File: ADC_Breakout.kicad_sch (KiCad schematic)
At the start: 38 parts, among them J0 Conn_01x06, J10 Conn_01x02, J11 Conn_01x02, J12 Conn_01x02, J13 Conn_01x02, J2 Digital Power, J3 Clock Chooser, J4 Analog Power, J6 Conn_01x02, J7 Conn_01x02, J8 Conn_01x02, J9 Conn_01x02, SW1 SW_MEC_5E, U2 SN74AUP2G80DCUR, X1 SIT8924BA-22-33E-8.192000, Y1 Crystal_Small

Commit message: Updated footprint.
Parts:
- D0: footprint Capacitor_SMD:C_0603_1608Metric_Pad1.08x0.95mm_HandSolder -> TVS:VAR_CG0603MLU-3.3E
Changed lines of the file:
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@@
 			)
 		)
-		(property "Footprint" "Capacitor_SMD:C_0603_1608Metric_Pad1.08x0.95mm_HandSolder"
+		(property "Footprint" "TVS:VAR_CG0603MLU-3.3E"
 			(at 38.1 88.9 0)
 			(effects

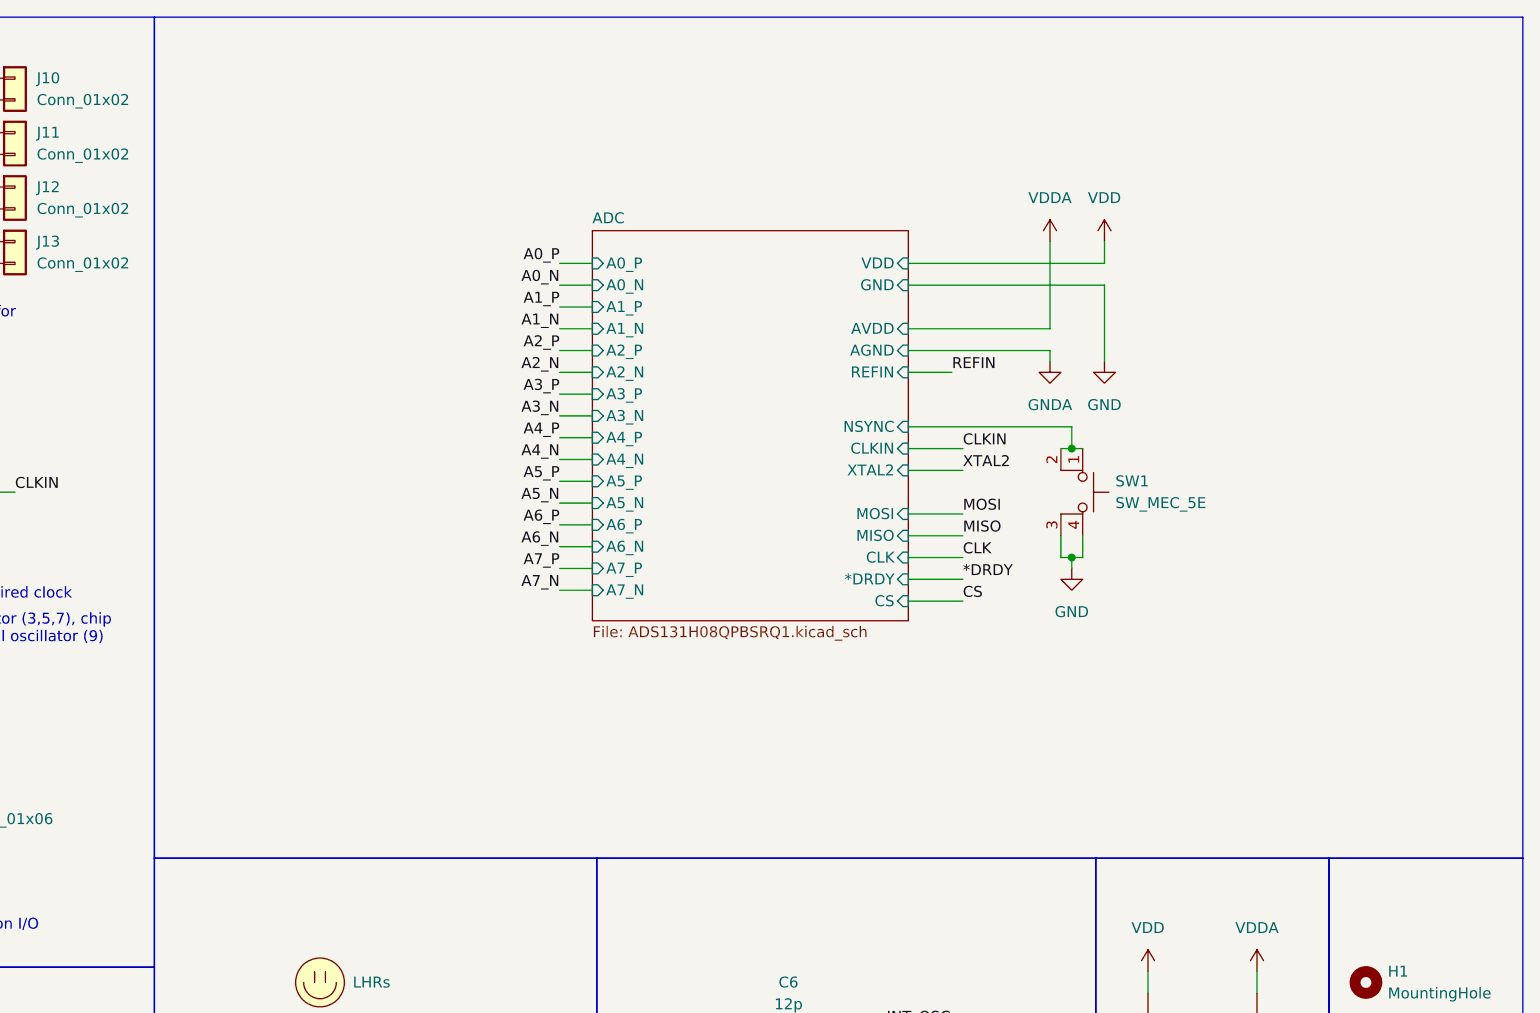
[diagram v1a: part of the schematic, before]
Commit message: gerebres
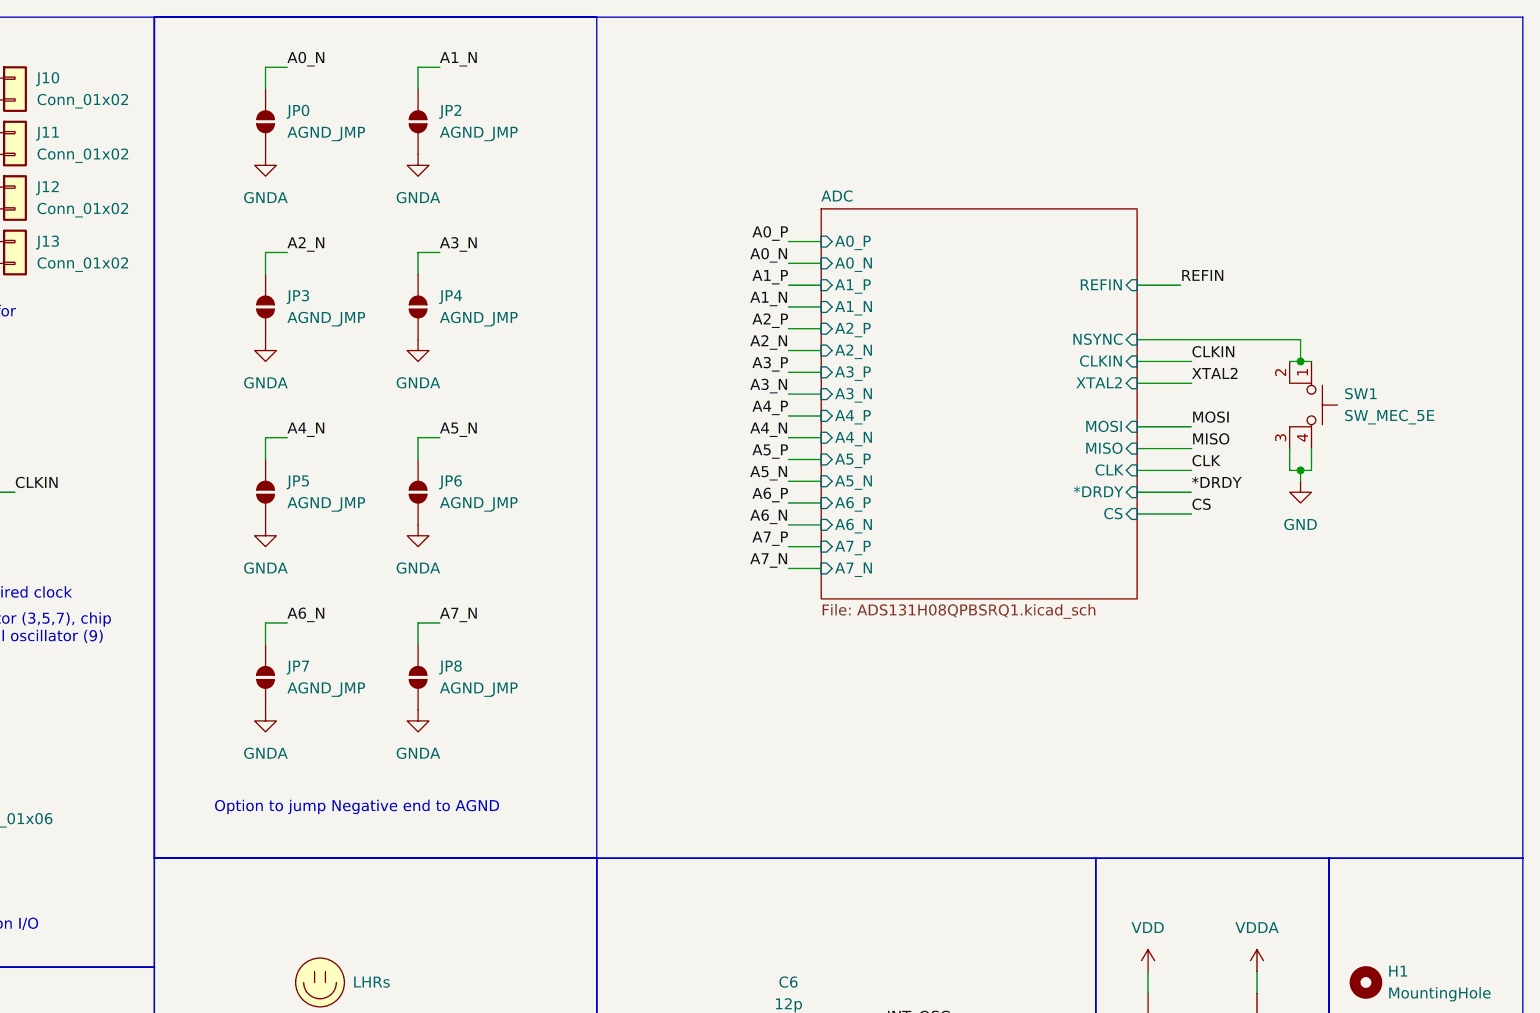
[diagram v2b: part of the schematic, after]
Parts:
- added JP0, JP2, JP3, JP4, JP5, JP6, JP7, JP8: AGND_JMP, Jumper:SolderJumper-2_P1.3mm_Open_TrianglePad1.0x1.5mm, symbol Jumper:SolderJumper_2_Open
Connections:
- net A0_N: now also JP0.1 (A)
- net A1_N: now also JP2.1 (A)
- net A2_N: now also JP3.1 (A)
- net A3_N: now also JP4.1 (A)
- net A4_N: now also JP5.1 (A)
- net A5_N: now also JP6.1 (A)
- net A6_N: now also JP7.1 (A)
- net A7_N: now also JP8.1 (A)
- net GNDA: now also JP0.2 (B), JP2.2 (B), JP3.2 (B), JP4.2 (B), JP5.2 (B), JP6.2 (B), JP7.2 (B), JP8.2 (B)
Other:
- sheet ADC ports: added none; removed AGND, AVDD, GND, VDD
- note added: "Option to jump Negative end to AGND"
- moved on the sheet: SW1
